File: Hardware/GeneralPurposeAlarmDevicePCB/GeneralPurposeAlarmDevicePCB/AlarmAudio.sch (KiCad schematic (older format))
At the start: 12 parts, among them J601 22-23-2021, Q601 MMBT2222A-7-F, Q602 MMBT2907ALT1G

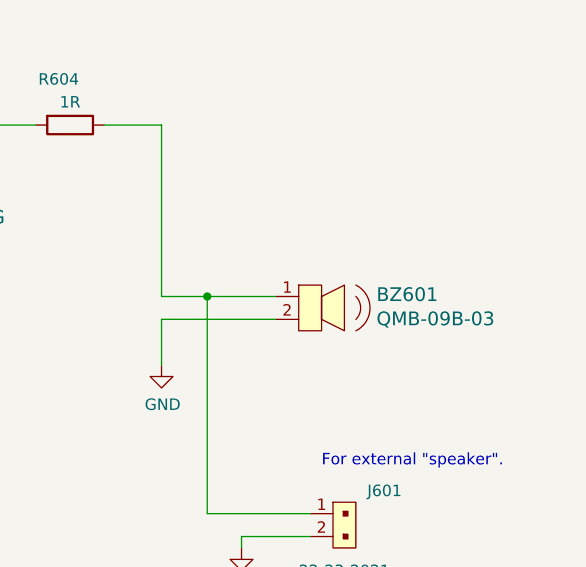
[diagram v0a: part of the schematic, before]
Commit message: Still have to make a 3D for buzzer and for USB connector. Still have to make PubInv logo and other Open Source logos. Experimental PCB placement tightned up.
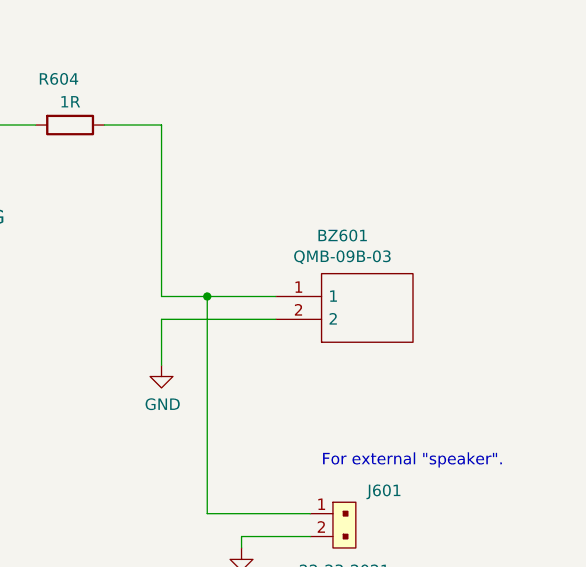
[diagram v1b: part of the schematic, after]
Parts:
- removed BZ601: QMB-09B-03, GeneralPurposeAlarmDevicePCB:MagneticBuzzer_9mmx5.8mmP=4mm, symbol GPAD_SCH_LIB:QMB-09B-03
- added BZ601: QMB-09B-03, QMB-09B-03:QMB09B03, symbol QMB-09B-03:QMB-09B-03
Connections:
- net GND: now also BZ601.2
- net at J601.1, R604.1: now also BZ601.1
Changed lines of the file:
@@
 $EndComp
-Wire Wire Line
-	7400 3550 6900 3550
 Wire Wire Line
 	6900 3550 6900 3750
@@
 	3400 3550 3750 3550
 $Comp
-L GPAD_SCH_LIB:QMB-09B-03 BZ601
-U 1 1 63A1E0DF
-P 7500 3550
-F 0 "BZ601" H 7840 3658 60  0000 L CNN
-F 1 "QMB-09B-03" H 7840 3552 60  0000 L CNN
-F 2 "GeneralPurposeAlarmDevicePCB:MagneticBuzzer_9mmx5.8mmP=4mm" H 7700 3750 60  0001 L CNN
-F 3 "2104011834_Jiangsu-Huaneng-Elec-QMB-09B-03_C96256.pdf" H 7700 3850 60  0001 L CNN
-F 4 "" H 7700 3950 60  0001 L CNN "Digi-Key_PN"
-F 5 "QMB-09B-03" H 7700 4050 60  0001 L CNN "MPN"
-F 6 "Audio Products" H 7700 4150 60  0001 L CNN "Category"
-F 7 "Alarms, Buzzers, and Sirens" H 7700 4250 60  0001 L CNN "Family"
-F 8 "https://www.murata.com/~/media/webrenewal/products/sound/sounder/vppt-buzj083-d.ashx" H 7700 4350 60  0001 L CNN "DK_Datasheet_Link"
-F 9 "/product-detail/en/murata-electronics-north-america/PKMCS0909E4000-R1/490-9647-1-ND/4878401" H 7700 4450 60  0001 L CNN "DK_Detail_Page"
-F 10 "5.7mm 9mm Externally Driven 85dB@3V,10cm 2V~5V Magnetic 3V 2700Hz Plugin,P=4mm Buzzers ROHS" H 7700 4550 60  0001 L CNN "Description"
-F 11 "Jiangsu Huaneng Elec" H 7700 4650 60  0001 L CNN "Manufacturer"
-F 12 "Active" H 7700 4750 60  0001 L CNN "Status"
-F 13 "JLCPCB" H 7500 3550 50  0001 C CNN "Distirbutor 1"
-F 14 "C96256" H 7500 3550 50  0001 C CNN "Distirbutor 1 PN"
-	1    7500 3550
-	1    0    0    -1
-$EndComp
-$Comp
 L Device:R R?
 U 1 1 63A4299B
@@
 	0    1    1    0
 $EndComp
+Wire Wire Line
+	7400 3550 6900 3550
+$Comp
+L QMB-09B-03:QMB-09B-03 BZ601
+U 1 1 62CCB6C9
+P 7400 3550
+F 0 "BZ601" H 7692 3185 50  0000 C CNN
+F 1 "QMB-09B-03" H 7692 3276 50  0000 C CNN
+F 2 "QMB-09B-03:QMB09B03" H 8050 3650 50  0001 L CNN
+F 3 "https://datasheet.lcsc.com/szlcsc/Jiangsu-Huaneng-Elec-QMB-09B-03_C96256.pdf" H 8050 3550 50  0001 L CNN
+F 4 "Magnetic NO 2700Hz 3V 2 ~ 5V 9mm 9*5.5mm Buzzers" H 8050 3450 50  0001 L CNN "Description"
+F 5 "Jiangsu Huaneng Elec" H 8050 3250 50  0001 L CNN "Manufacturer"
+F 6 "QMB-09B-03" H 8050 3150 50  0001 L CNN "MPN"
+F 7 "JLCPCB" H 7400 3550 50  0001 C CNN "Distributor 1"
+F 8 "C96256" H 7400 3550 50  0001 C CNN "Distributor 1 PN"
+	1    7400 3550
+	1    0    0    1
+$EndComp
 $EndSCHEMATC
